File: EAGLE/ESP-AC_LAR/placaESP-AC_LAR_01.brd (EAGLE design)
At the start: 42.5 x 44.5 mm, 15 parts, among them Q1 2N4401, X1 22-23-2021

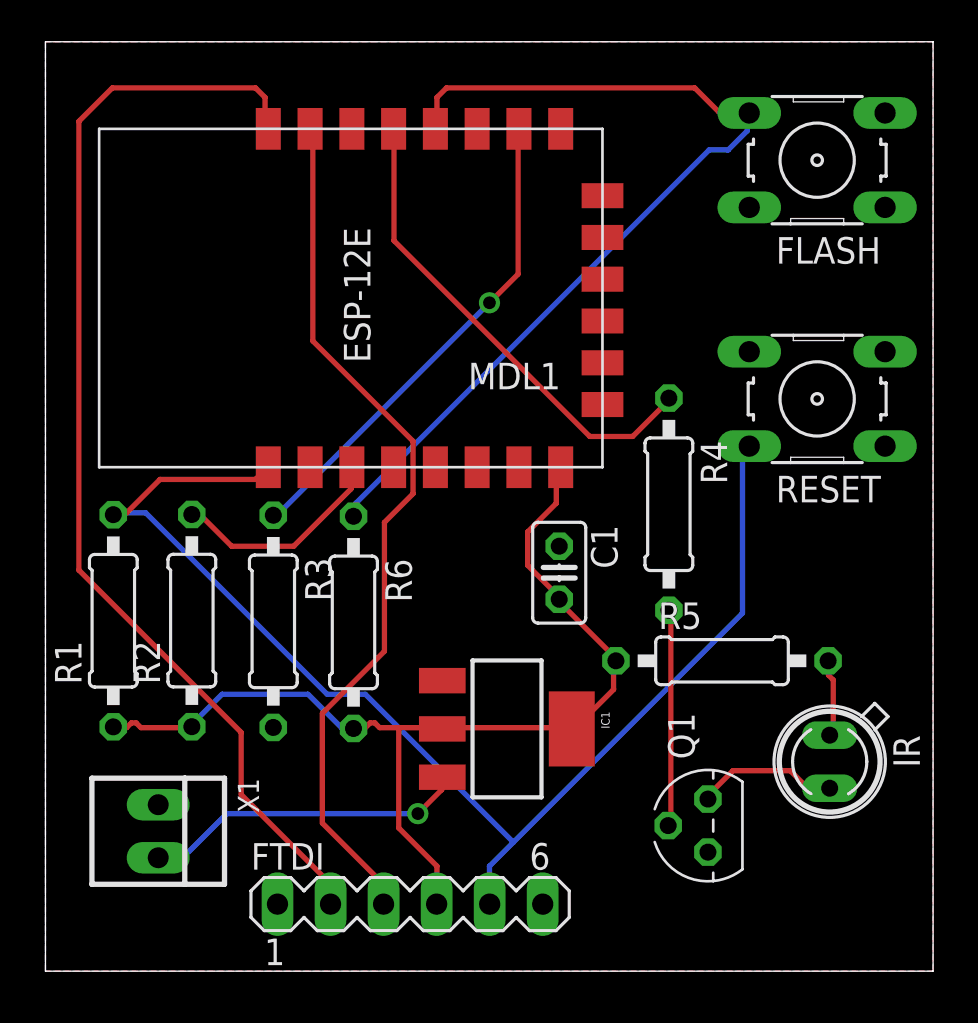
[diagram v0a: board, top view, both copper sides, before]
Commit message: Add gerbers + atualização caixa
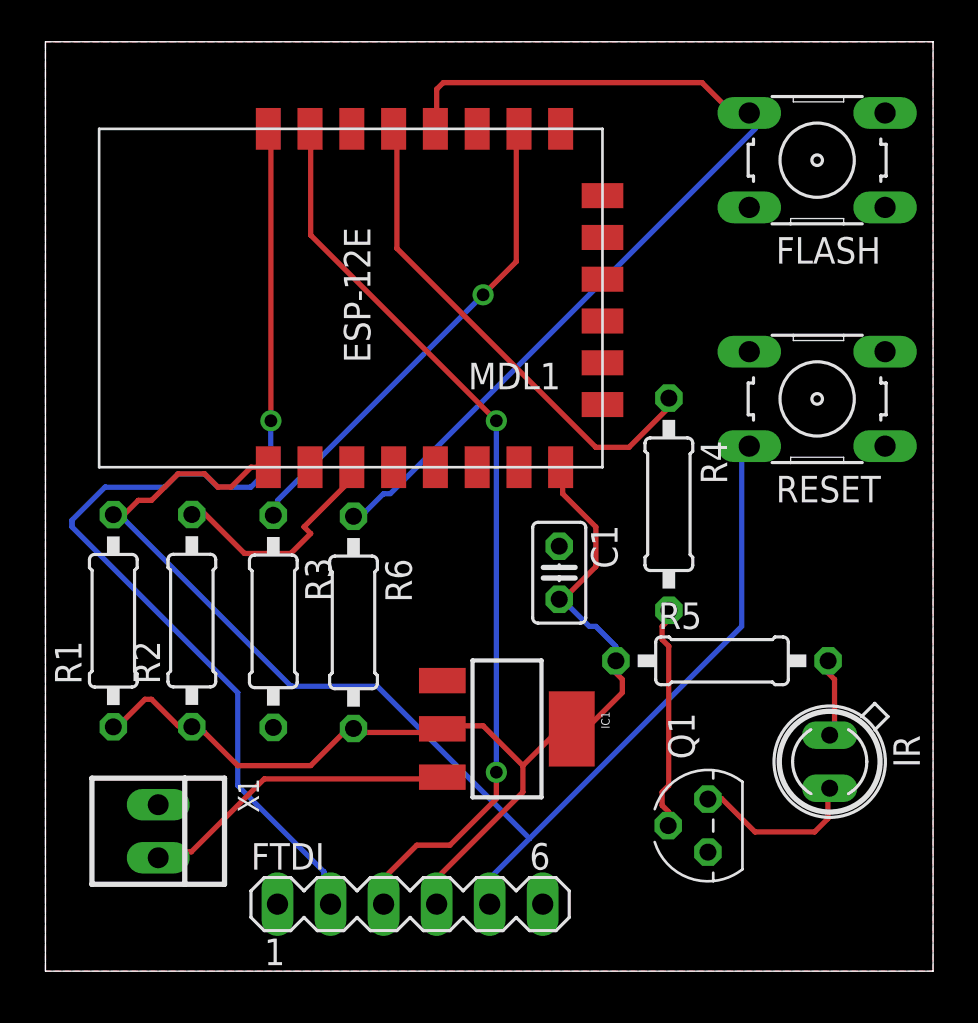
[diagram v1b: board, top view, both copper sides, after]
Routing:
- net RXI: track 53.8 -> 50.9 mm, vias 0 -> 1
- net VCC: track 49.2 -> 52.0 mm
- net TXO: track 42.2 -> 44.0 mm, vias 0 -> 2
- net CTS: track 61.1 -> 62.5 mm
- net N$4: track 6.86 -> 8.14 mm
- net IO4: track 23.4 -> 24.4 mm
- net N$1: track 10.5 -> 11.5 mm
- net N$3: track 10.4 -> 11.2 mm
- net N$6: track 44.8 -> 45.5 mm
- net IN+: track 15.5 -> 15.2 mm, vias 1 -> 0
